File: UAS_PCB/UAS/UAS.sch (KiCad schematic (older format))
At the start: 17 parts, among them J1 SM02B-PASS-TBT, J2 SM02B-PASS-TBT, J3 SM02B-PASS-TBT, J4 SM02B-PASS-TBT, U1 JST-7-Pin, U10 UAS-rescue_7.5V-2.4A-Converte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, U11 JST-3-Pin, U12 Signal-Pad, U13 Signal-Pad, U2 5A-5V-Converter, U3 500mA-5V-Converter, U4 12V-StepUp-Converter, U5 TB6612FNG-Dual-Motor-Driver, U6 16_Pad_2x8_Set-UAS-cache, U7 UAS-rescue_JST-4-Pin-UAS-cache, U8 JST-7-Pin, U9 JST-3-Pin

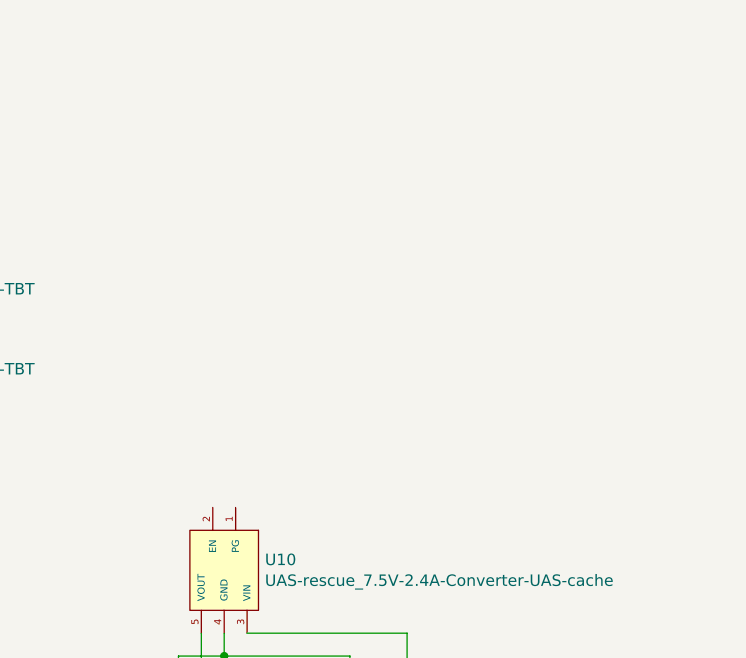
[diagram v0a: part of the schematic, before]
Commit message: final version with kyles passthrough pads and graphics
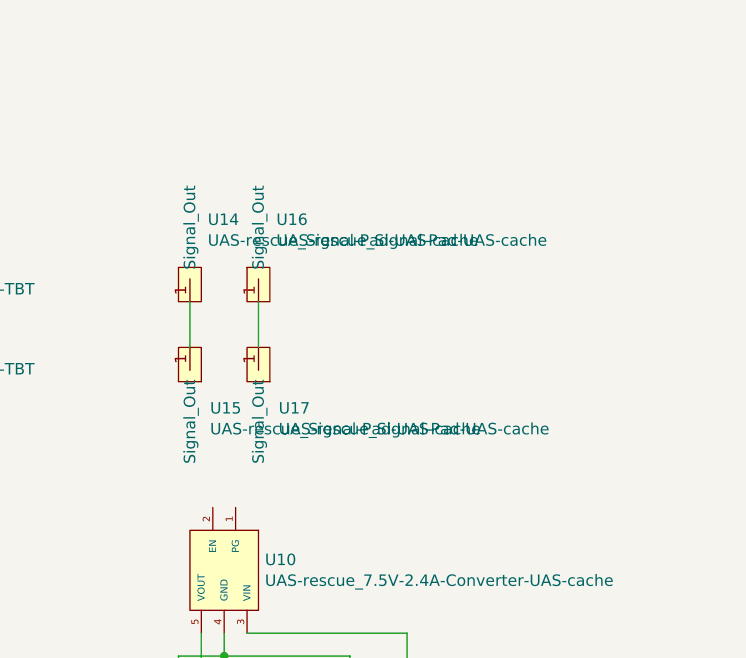
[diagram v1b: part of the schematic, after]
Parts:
- added U14, U15, U16, U17: UAS-rescue_Signal-Pad-UAS-cache, UAS:Individual_Solder_Pad, symbol UAS-cache:UAS-rescue_Signal-Pad-UAS-cache
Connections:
- new net: U14.1 (Signal_Out), U15.1 (Signal_Out)
- new net: U16.1 (Signal_Out), U17.1 (Signal_Out)
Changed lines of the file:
@@
 Wire Wire Line
 	2800 3650 2800 3900
+$Comp
+L UAS-cache:UAS-rescue_Signal-Pad-UAS-cache U17
+U 1 1 603DAF7F
+P 5600 3750
+F 0 "U17" H 5512 3916 50  0000 R CNN
+F 1 "UAS-rescue_Signal-Pad-UAS-cache" H 5512 4007 50  0000 R CNN
+F 2 "UAS:Individual_Solder_Pad" H 5600 3750 50  0001 C CNN
+F 3 "" H 5600 3750 50  0001 C CNN
+	1    5600 3750
+	-1   0    0    1
+$EndComp
+$Comp
+L UAS-cache:UAS-rescue_Signal-Pad-UAS-cache U15
+U 1 1 603D9E61
+P 5300 3750
+F 0 "U15" H 5212 3916 50  0000 R CNN
+F 1 "UAS-rescue_Signal-Pad-UAS-cache" H 5212 4007 50  0000 R CNN
+F 2 "UAS:Individual_Solder_Pad" H 5300 3750 50  0001 C CNN
+F 3 "" H 5300 3750 50  0001 C CNN
+	1    5300 3750
+	-1   0    0    1
+$EndComp
+$Comp
+L UAS-cache:UAS-rescue_Signal-Pad-UAS-cache U16
+U 1 1 603D9324
+P 5600 3350
+F 0 "U16" H 5678 3609 50  0000 L CNN
+F 1 "UAS-rescue_Signal-Pad-UAS-cache" H 5678 3518 50  0000 L CNN
+F 2 "UAS:Individual_Solder_Pad" H 5600 3350 50  0001 C CNN
+F 3 "" H 5600 3350 50  0001 C CNN
+	1    5600 3350
+	1    0    0    -1
+$EndComp
+$Comp
+L UAS-cache:UAS-rescue_Signal-Pad-UAS-cache U14
+U 1 1 603D8772
+P 5300 3350
+F 0 "U14" H 5378 3609 50  0000 L CNN
+F 1 "UAS-rescue_Signal-Pad-UAS-cache" H 5378 3518 50  0000 L CNN
+F 2 "UAS:Individual_Solder_Pad" H 5300 3350 50  0001 C CNN
+F 3 "" H 5300 3350 50  0001 C CNN
+	1    5300 3350
+	1    0    0    -1
+$EndComp
+Wire Wire Line
+	5300 3450 5300 3650
+Wire Wire Line
+	5600 3450 5600 3650
 $EndSCHEMATC
